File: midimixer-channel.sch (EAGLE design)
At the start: 94 parts, among them IC1 74LS595D, IC2 74LS595D, IC3 74LS595D, IC4 74LS595D, U1 LM1117IMPX-3.3/NOPB, Y1 8MHz 695-HCM49-8-U

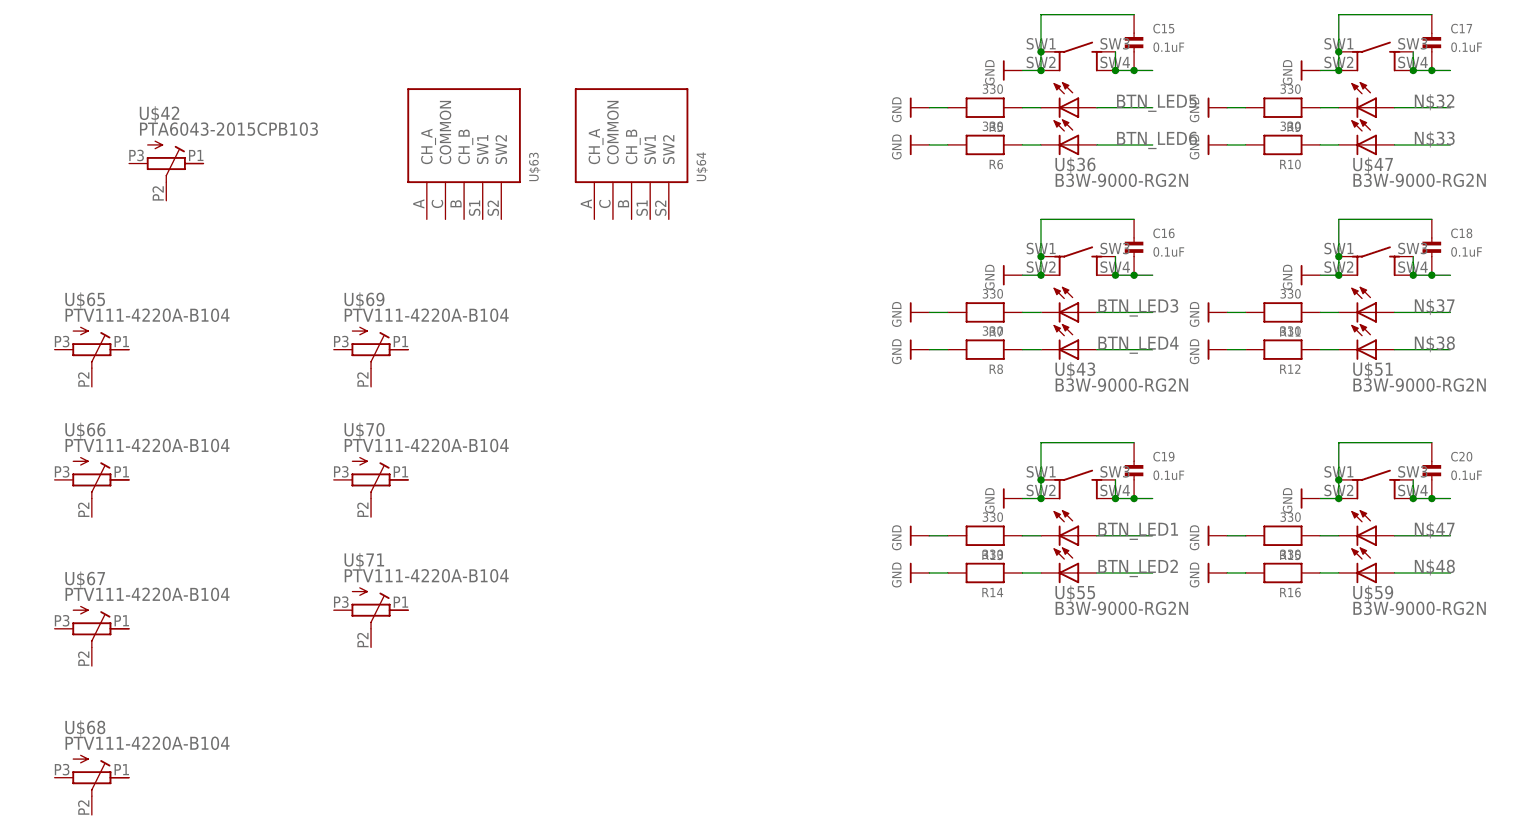
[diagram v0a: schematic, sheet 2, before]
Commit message: wip
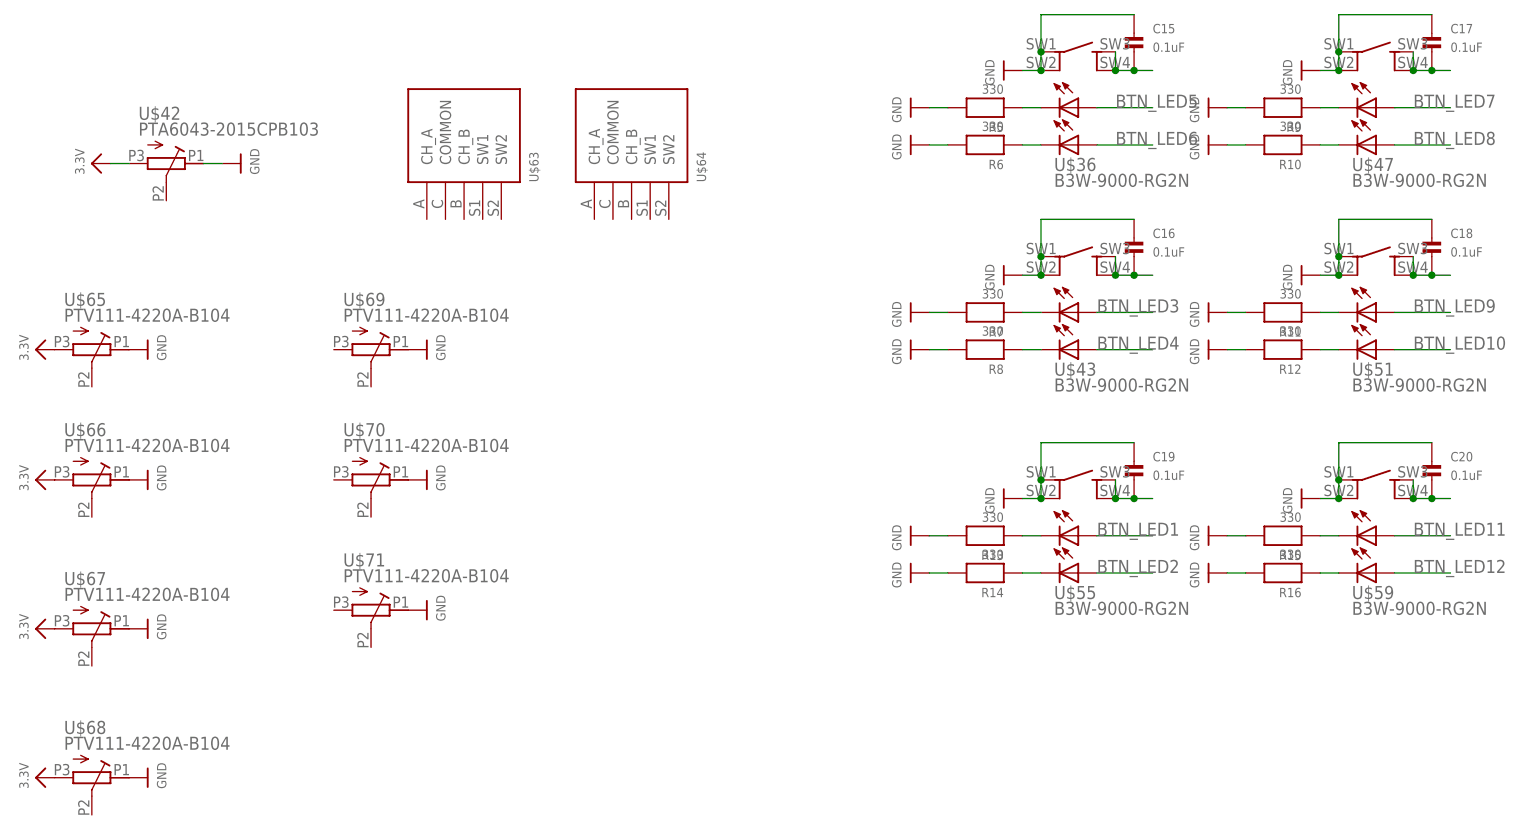
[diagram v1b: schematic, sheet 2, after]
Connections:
- removed net N$32: U$47.LED1+
- removed net N$33: U$47.LED2+
- removed net N$37: U$51.LED1+
- removed net N$38: U$51.LED2+
- removed net N$47: U$59.LED1+
- removed net N$48: U$59.LED2+
- net 3.3V: now also U$42.E, U$65.E, U$66.E, U$67.E, U$68.E
- net BTN_LED10: now also U$51.LED2+
- net BTN_LED11: now also U$59.LED1+
- net BTN_LED12: now also U$59.LED2+
- net BTN_LED7: now also U$47.LED1+
- net BTN_LED8: now also U$47.LED2+
- net BTN_LED9: now also U$51.LED1+
- net GND: now also U$42.A, U$65.A, U$66.A, U$67.A, U$68.A, U$69.A, U$70.A, U$71.A
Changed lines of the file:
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@@
 <part name="U$96" library="microbuilder" deviceset="GND" device=""/>
 <part name="R27" library="microbuilder" deviceset="RESISTOR" device="_0603" value="120"/>
+<part name="U$97" library="microbuilder" deviceset="GND" device=""/>
+<part name="U$98" library="microbuilder" deviceset="3.3V" device=""/>
+<part name="U$99" library="microbuilder" deviceset="GND" device=""/>
+<part name="U$100" library="microbuilder" deviceset="GND" device=""/>
+<part name="U$101" library="microbuilder" deviceset="GND" device=""/>
+<part name="U$102" library="microbuilder" deviceset="GND" device=""/>
+<part name="U$103" library="microbuilder" deviceset="GND" device=""/>
+<part name="U$104" library="microbuilder" deviceset="GND" device=""/>
+<part name="U$105" library="microbuilder" deviceset="GND" device=""/>
+<part name="U$106" library="microbuilder" deviceset="3.3V" device=""/>
+<part name="U$107" library="microbuilder" deviceset="3.3V" device=""/>
+<part name="U$108" library="microbuilder" deviceset="3.3V" device=""/>
+<part name="U$109" library="microbuilder" deviceset="3.3V" device=""/>
 </parts>
 <sheets>
@@
 <instance part="U$70" gate="G$1" x="45.72" y="-30.48" rot="R270"/>
 <instance part="U$71" gate="G$1" x="45.72" y="-48.26" rot="R270"/>
+<instance part="U$97" gate="G$1" x="27.94" y="12.7" rot="R90"/>
+<instance part="U$98" gate="G$1" x="7.62" y="12.7" rot="R90"/>
+<instance part="U$99" gate="G$1" x="53.34" y="-12.7" rot="R90"/>
+<instance part="U$100" gate="G$1" x="53.34" y="-30.48" rot="R90"/>
+<instance part="U$101" gate="G$1" x="53.34" y="-48.26" rot="R90"/>
+<instance part="U$102" gate="G$1" x="15.24" y="-71.12" rot="R90"/>
+<instance part="U$103" gate="G$1" x="15.24" y="-50.8" rot="R90"/>
+<instance part="U$104" gate="G$1" x="15.24" y="-30.48" rot="R90"/>
+<instance part="U$105" gate="G$1" x="15.24" y="-12.7" rot="R90"/>
+<instance part="U$106" gate="G$1" x="0" y="-12.7" rot="R90"/>
+<instance part="U$107" gate="G$1" x="0" y="-30.48" rot="R90"/>
+<instance part="U$108" gate="G$1" x="0" y="-50.8" rot="R90"/>
+<instance part="U$109" gate="G$1" x="0" y="-71.12" rot="R90"/>
 </instances>
 <busses>
@@
 <junction x="177.8" y="-30.48"/>
 </segment>
+<segment>
+<pinref part="U$42" gate="G$1" pin="A"/>
+<pinref part="U$97" gate="G$1" pin="GND"/>
+<wire x1="25.4" y1="12.7" x2="22.86" y2="12.7" width="0.1524" layer="91"/>
+</segment>
+<segment>
+<pinref part="U$69" gate="G$1" pin="A"/>
+<pinref part="U$99" gate="G$1" pin="GND"/>
+</segment>
+<segment>
+<pinref part="U$70" gate="G$1" pin="A"/>
+<pinref part="U$100" gate="G$1" pin="GND"/>
+</segment>
+<segment>
+<pinref part="U$71" gate="G$1" pin="A"/>
+<pinref part="U$101" gate="G$1" pin="GND"/>
+</segment>
+<segment>
+<pinref part="U$68" gate="G$1" pin="A"/>
+<pinref part="U$102" gate="G$1" pin="GND"/>
+</segment>
+<segment>
+<pinref part="U$67" gate="G$1" pin="A"/>
+<pinref part="U$103" gate="G$1" pin="GND"/>
+</segment>
+<segment>
+<pinref part="U$66" gate="G$1" pin="A"/>
+<pinref part="U$104" gate="G$1" pin="GND"/>
+</segment>
+<segment>
+<pinref part="U$65" gate="G$1" pin="A"/>
+<pinref part="U$105" gate="G$1" pin="GND"/>
+</segment>
 </net>
 <net name="N$9" class="0">
@@
 </segment>
 </net>
-<net name="N$32" class="0">
+<net name="BTN_LED7" class="0">
 <segment>
 <pinref part="U$47" gate="G$1" pin="LED1+"/>
@@
 </segment>
 </net>
-<net name="N$33" class="0">
+<net name="BTN_LED8" class="0">
 <segment>
 <pinref part="U$47" gate="G$1" pin="LED2+"/>
@@
 </segment>
 </net>
-<net name="N$37" class="0">
+<net name="BTN_LED9" class="0">
 <segment>
 <pinref part="U$51" gate="G$1" pin="LED1+"/>
@@
 </segment>
 </net>
-<net name="N$38" class="0">
+<net name="BTN_LED10" class="0">
 <segment>
 <pinref part="U$51" gate="G$1" pin="LED2+"/>
@@
 </segment>
 </net>
-<net name="N$47" class="0">
+<net name="BTN_LED11" class="0">
 <segment>
 <pinref part="U$59" gate="G$1" pin="LED1+"/>
@@
 </segment>
 </net>
-<net name="N$48" class="0">
+<net name="BTN_LED12" class="0">
 <segment>
 <pinref part="U$59" gate="G$1" pin="LED2+"/>
@@
 </segment>
 </net>
+<net name="3.3V" class="0">
+<segment>
+<pinref part="U$42" gate="G$1" pin="E"/>
+<pinref part="U$98" gate="G$1" pin="3.3V"/>
+<wire x1="10.16" y1="12.7" x2="12.7" y2="12.7" width="0.1524" layer="91"/>
+</segment>
+<segment>
+<pinref part="U$65" gate="G$1" pin="E"/>
+<pinref part="U$106" gate="G$1" pin="3.3V"/>
+</segment>
+<segment>
+<pinref part="U$66" gate="G$1" pin="E"/>
+<pinref part="U$107" gate="G$1" pin="3.3V"/>
+</segment>
+<segment>
+<pinref part="U$67" gate="G$1" pin="E"/>
+<pinref part="U$108" gate="G$1" pin="3.3V"/>
+</segment>
+<segment>
+<pinref part="U$68" gate="G$1" pin="E"/>
+<pinref part="U$109" gate="G$1" pin="3.3V"/>
+</segment>
+</net>
